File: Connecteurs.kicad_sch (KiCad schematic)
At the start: 22 parts, among them J10 DZ254S-11-02-48, J11 DZ254S-11-02-48, J2 GT-USB-7002A, J3 BH127VS-14P-H49, Q7 AO3401A

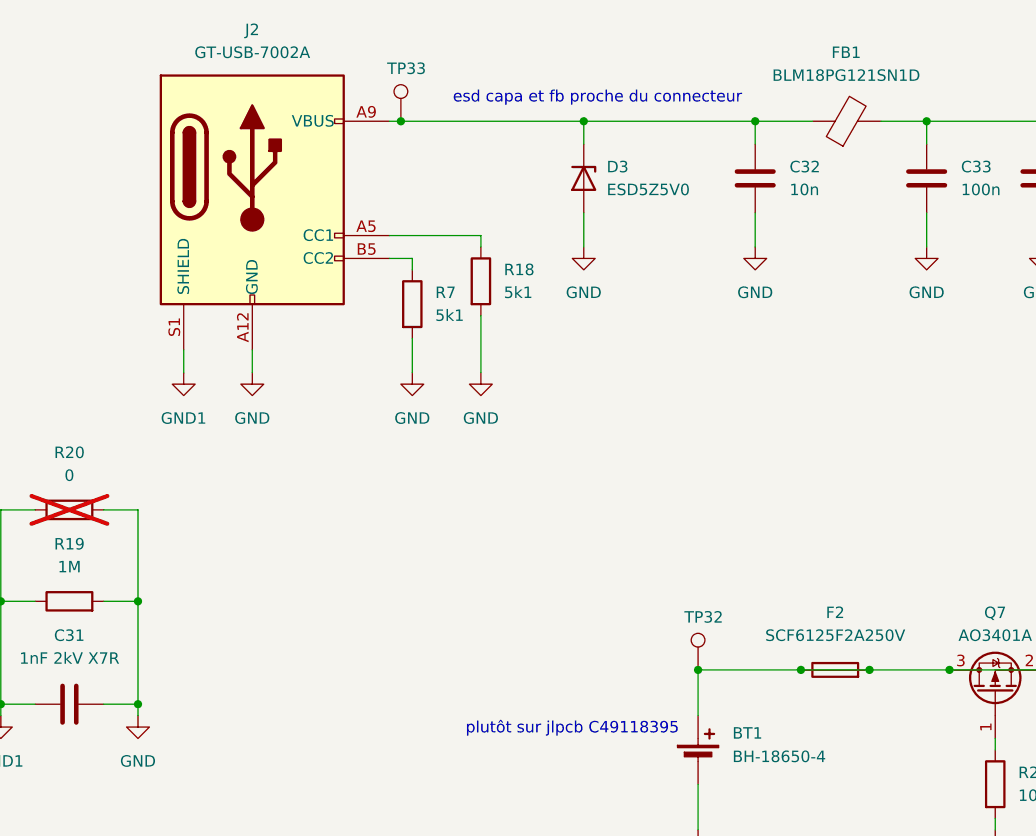
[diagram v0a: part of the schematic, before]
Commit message: t
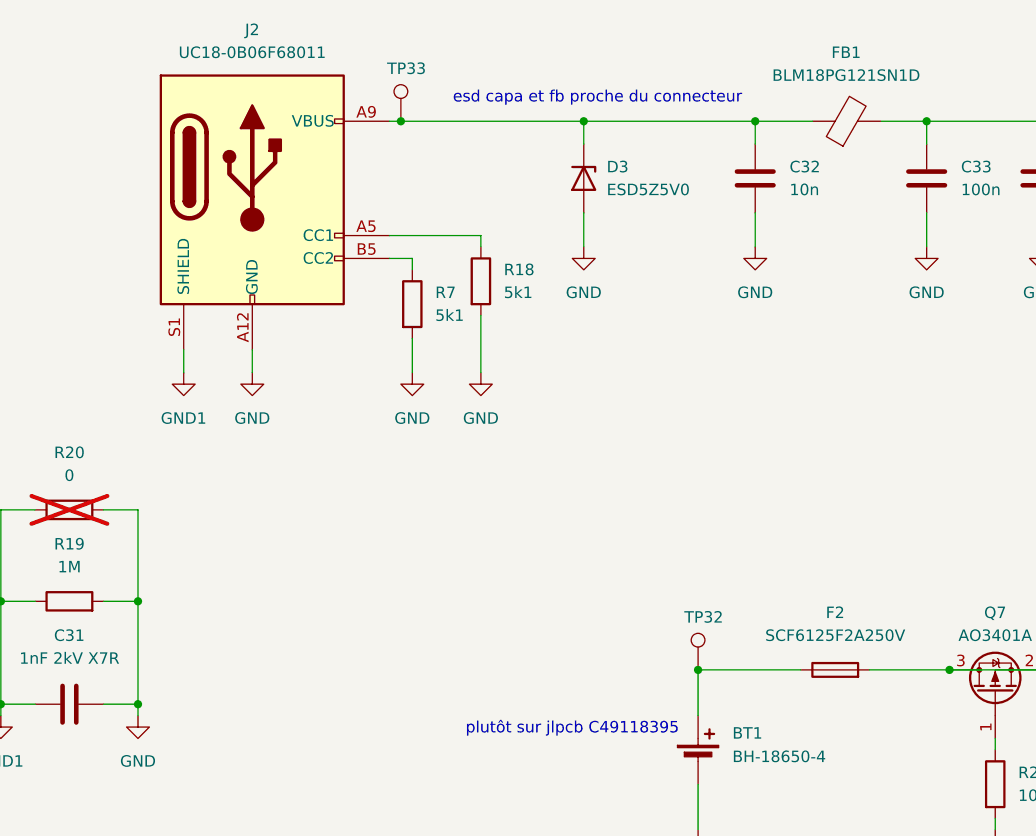
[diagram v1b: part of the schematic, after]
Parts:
- J2: value GT-USB-7002A -> UC18-0B06F68011; LCSC C963365 -> C36936555
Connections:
- net at D7.1 (K), F2.2, J11.2 (Pin_2)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: no longer BT1.1 (+), F2.1, TP32.1
- new net: BT1.1 (+), F2.1, TP32.1
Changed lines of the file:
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@@
-	)
-	(junction
-		(at 118.11 97.79)
-		(diameter 0)
-		(color 0 0 0 0)
 	)
 	(junction
@@
 	)
 	(junction
-		(at 125.73 97.79)
-		(diameter 0)
-		(color 0 0 0 0)
-	)
-	(junction
 		(at 44.45 101.6)
 		(diameter 0)
@@
 		(pts
 			(xy 166.37 92.71) (xy 166.37 97.79)
-		)
-		(stroke
-			(width 0)
-			(type default)
-		)
-	)
-	(wire
-		(pts
-			(xy 125.73 97.79) (xy 118.11 97.79)
 		)
 		(stroke
@@
 			)
 		)
-		(property "Value" "GT-USB-7002A"
+		(property "Value" "UC18-0B06F68011"
 			(at 57.15 29.21 0)
 			(effects
@@
 			)
 		)
-		(property "LCSC" "C963365"
+		(property "LCSC" "C36936555"
 			(at 57.15 44.45 0)
 			(effects

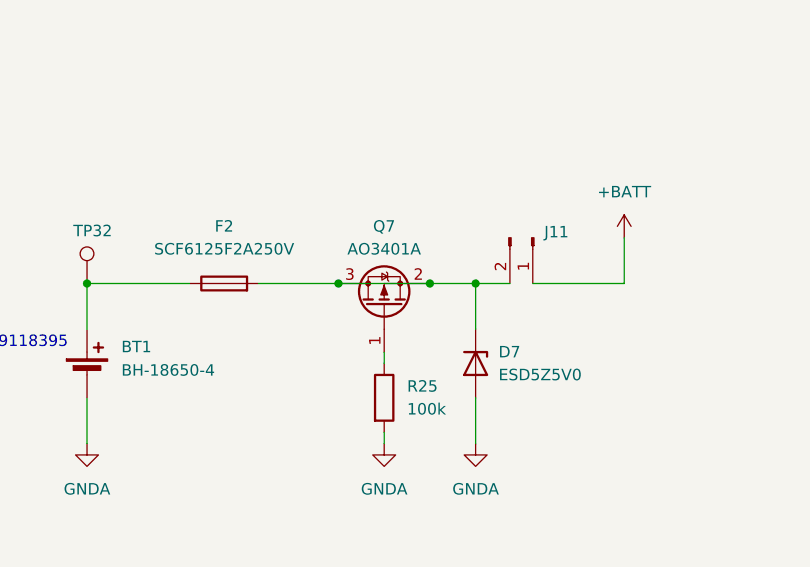
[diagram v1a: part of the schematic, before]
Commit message: V1 Placement + Routage
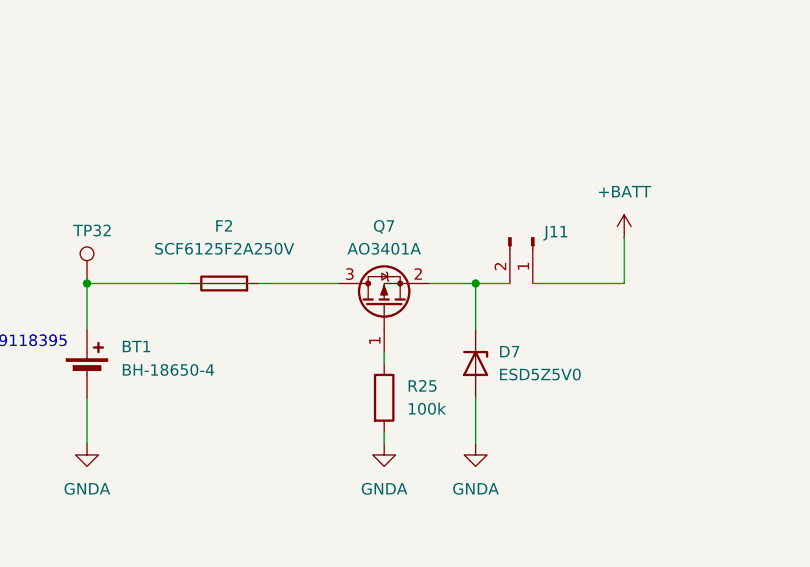
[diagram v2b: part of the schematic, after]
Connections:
- net at D7.1 (K), J11.2 (Pin_2), Q7.2 (S): no longer F2.2, Q7.3 (D)
- new net: F2.2, Q7.3 (D)
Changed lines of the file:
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@@
-	)
-	(junction
-		(at 144.78 97.79)
-		(diameter 0)
-		(color 0 0 0 0)
 	)
 	(junction
@@
 	)
 	(junction
+		(at 149.86 97.79)
+		(diameter 0)
+		(color 0 0 0 0)
+	)
+	(junction
 		(at 44.45 101.6)
 		(diameter 0)
@@
 	)
 	(junction
-		(at 149.86 97.79)
-		(diameter 0)
-		(color 0 0 0 0)
-	)
-	(junction
-		(at 134.62 97.79)
-		(diameter 0)
-		(color 0 0 0 0)
-	)
-	(junction
 		(at 106.68 97.79)
 		(diameter 0)
@@
 	(wire
 		(pts
-			(xy 144.78 97.79) (xy 134.62 97.79)
-		)
-		(stroke
-			(width 0)
-			(type default)
-		)
-	)
-	(wire
-		(pts
 			(xy 180.34 36.83) (xy 180.34 33.02)
 		)
@@
 	(wire
 		(pts
-			(xy 149.86 97.79) (xy 144.78 97.79)
-		)
-		(stroke
-			(width 0)
-			(type default)
-		)
-	)
-	(wire
-		(pts
 			(xy 29.21 80.01) (xy 33.02 80.01)
 		)
@@
 	(wire
 		(pts
+			(xy 144.78 97.79) (xy 149.86 97.79)
+		)
+		(stroke
+			(width 0)
+			(type default)
+		)
+	)
+	(wire
+		(pts
 			(xy 214.63 41.91) (xy 207.01 41.91)
 		)
@@
 	(wire
 		(pts
+			(xy 125.73 97.79) (xy 134.62 97.79)
+		)
+		(stroke
+			(width 0)
+			(type default)
+		)
+	)
+	(wire
+		(pts
 			(xy 72.39 36.83) (xy 73.66 36.83)
 		)
 		(stroke
-			(width 0)
-			(type default)
-		)
-	)
-	(wire
-		(pts
-			(xy 125.73 97.79) (xy 134.62 97.79)
-		)
-		(stroke
